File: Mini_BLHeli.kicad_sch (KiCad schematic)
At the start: 2 parts

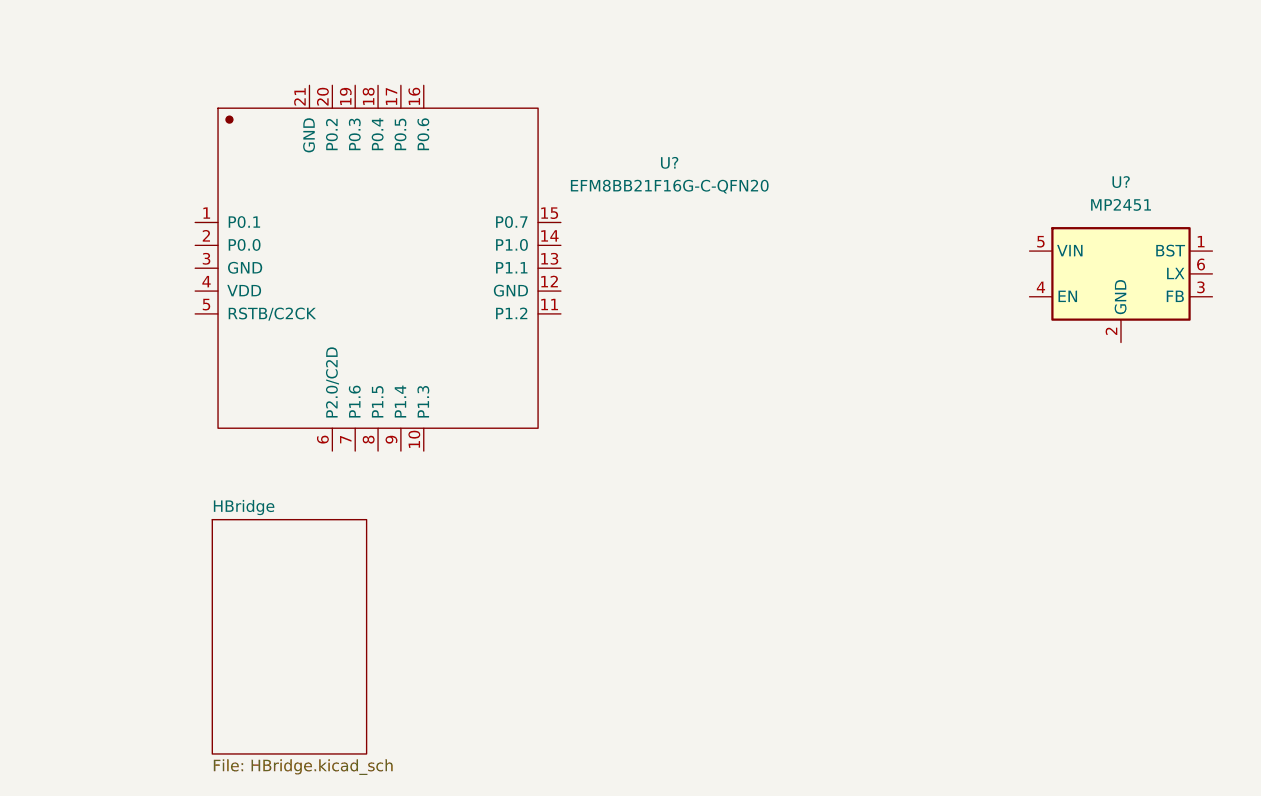
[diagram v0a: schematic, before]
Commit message: v0.9 finish
Signed-off-by: ncerzzk <huangzzk@bupt.edu.cn>
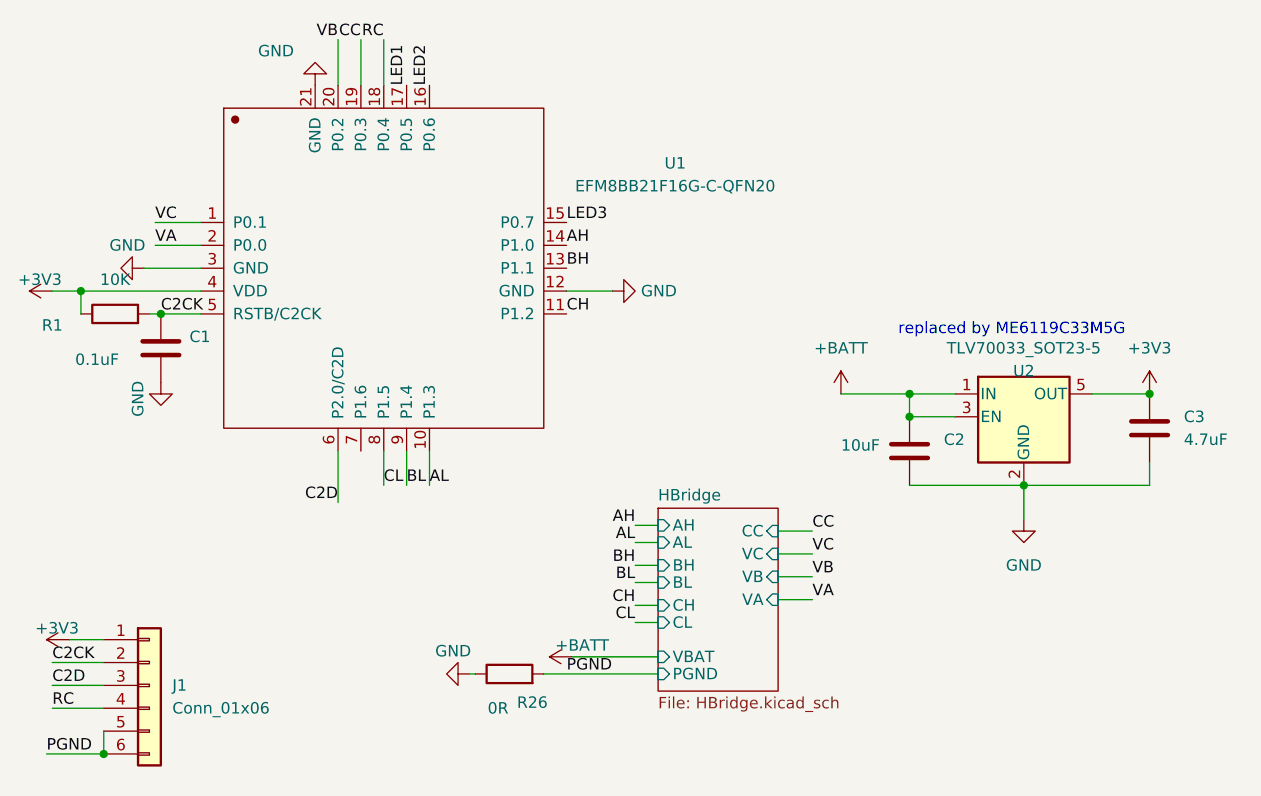
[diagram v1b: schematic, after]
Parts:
- removed U?: MP2451, Package_TO_SOT_SMD:SOT-23-6, symbol Regulator_Switching:AOZ1280CI
- added C1: 0.1uF, Capacitor_SMD:C_0402_1005Metric, symbol Device:C
- added C2: 10uF, Capacitor_SMD:C_0805_2012Metric, symbol Device:C
- added C3: 4.7uF, Capacitor_SMD:C_0402_1005Metric, symbol Device:C
- added J1: Conn_01x06, Connector_PinHeader_2.54mm:PinHeader_1x06_P2.54mm_Vertical, symbol Connector_Generic:Conn_01x06
- added R1: 10K, Resistor_SMD:R_0402_1005Metric, symbol Device:R
- added R26: 0R, Resistor_SMD:R_0402_1005Metric, symbol Device:R
- added U2: TLV70033_SOT23-5, Package_TO_SOT_SMD:SOT-23-5, symbol Regulator_Linear:TLV70033_SOT23-5
- U1: renamed from U?; footprint kicad_lceda:QFN-20_L3.0-W3.0-P0.50-BL-EP1.7_EFM8BB21F16G -> Package_DFN_QFN:SiliconLabs_QFN-20-1EP_3x3mm_P0.5mm_EP1.8x1.8mm
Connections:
- net VC: now reaches U1.1 (P0.1)
- net AL: now reaches U1.10 (P1.3)
- net CH: now reaches U1.11 (P1.2)
- net GND: now reaches U1.12 (GND)
- net GND: now also U1.21 (GND), U1.3 (GND), C1.2, C2.2, C3.2, R26.1, U2.2 (GND)
- net BH: now reaches U1.13 (P1.1)
- net AH: now reaches U1.14 (P1.0)
- net LED3: now reaches U1.15 (P0.7)
- net LED2: now reaches U1.16 (P0.6)
- net LED1: now reaches U1.17 (P0.5)
- net RC: now reaches U1.18 (P0.4)
- net RC: now also J1.4 (Pin_4)
- net CC: now reaches U1.19 (P0.3)
- net VA: now reaches U1.2 (P0.0)
- net VB: now reaches U1.20 (P0.2)
- net +3V3: now reaches U1.4 (VDD)
- net +3V3: now also C3.1, J1.1 (Pin_1), R1.1, U2.5 (OUT)
- net C2CK: now reaches U1.5 (RSTB/C2CK)
- net C2CK: now also C1.1, J1.2 (Pin_2), R1.2
- net C2D: now reaches U1.6 (P2.0/C2D)
- net C2D: now also J1.3 (Pin_3)
- net CL: now reaches U1.8 (P1.5)
- net BL: now reaches U1.9 (P1.4)
- new net +BATT: C2.1, U2.1 (IN), U2.3 (EN)
- new net PGND: J1.5 (Pin_5), J1.6 (Pin_6), R26.2
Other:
- sheet HBridge ports: added AH, AL, BH, BL, CC, CH, CL, PGND, VA, VB, VBAT, VC; removed none
- note added: "replaced by ME6119C33M5G"
- moved on the sheet: U1
